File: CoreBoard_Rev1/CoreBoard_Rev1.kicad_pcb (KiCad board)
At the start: 2 copper layers, 128.8 x 84.3 mm, 90 parts, among them J1 RJ45_LED_Shielded, SW1 SW_Push, SW10 SW_Push, SW11 SW_Push, SW12 SW_Push, SW13 SW_Push, SW14 SW_Push, SW15 SW_Push, SW16 SW_SPDT, SW2 SW_Push, SW3 SW_Push, SW4 SW_Push, SW5 SW_Push, SW6 SW_Push, SW7 SW_Push, SW8 SW_Push, SW9 SW_Push, U1 Teensy4.1_DEV-16771, U2 TSR_1-2450, U4 74HC148, U5 74HC148, U6 74HC00, U7 OKI

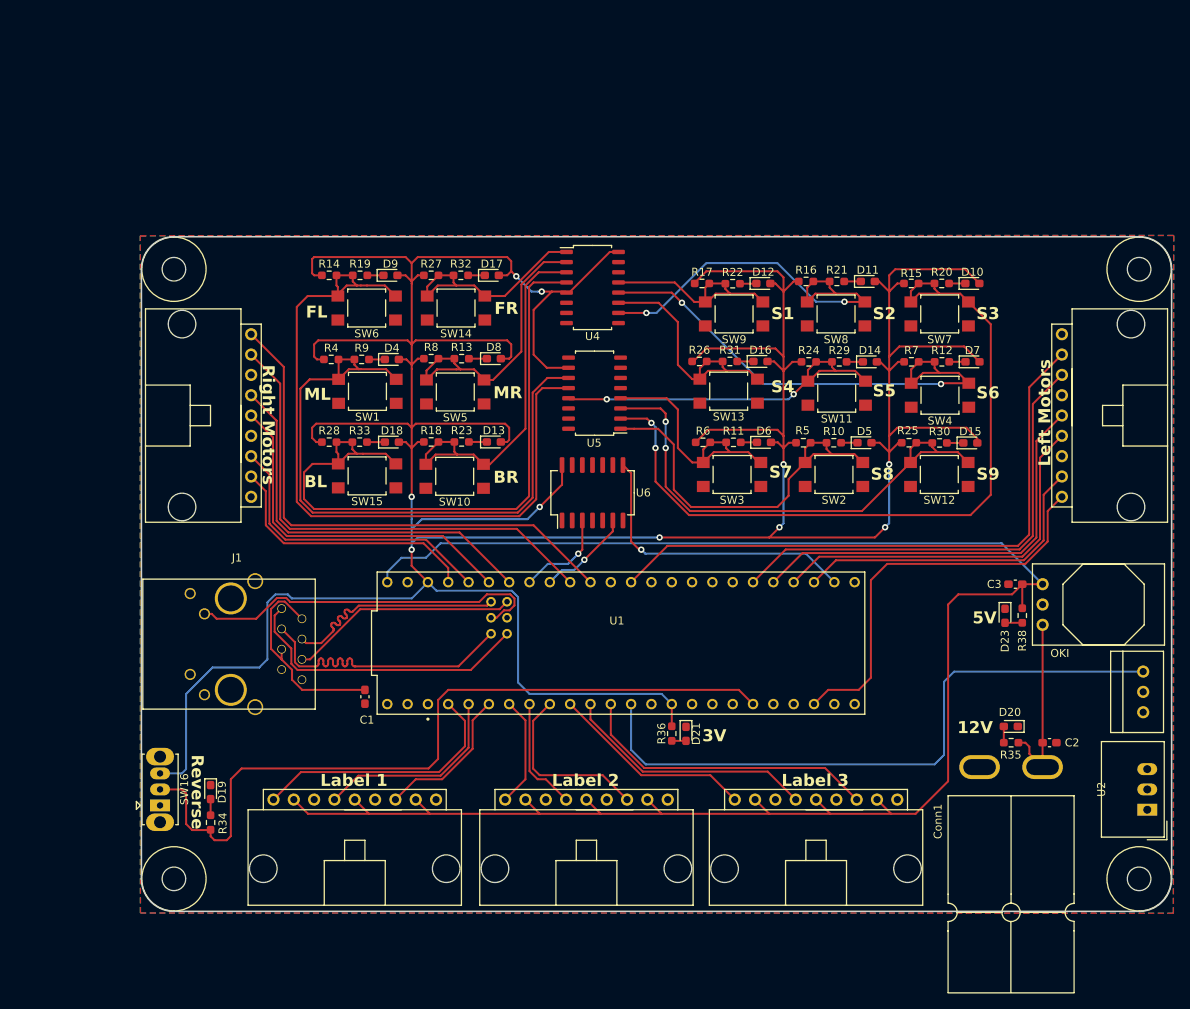
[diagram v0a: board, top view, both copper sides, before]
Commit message: connected remaining components
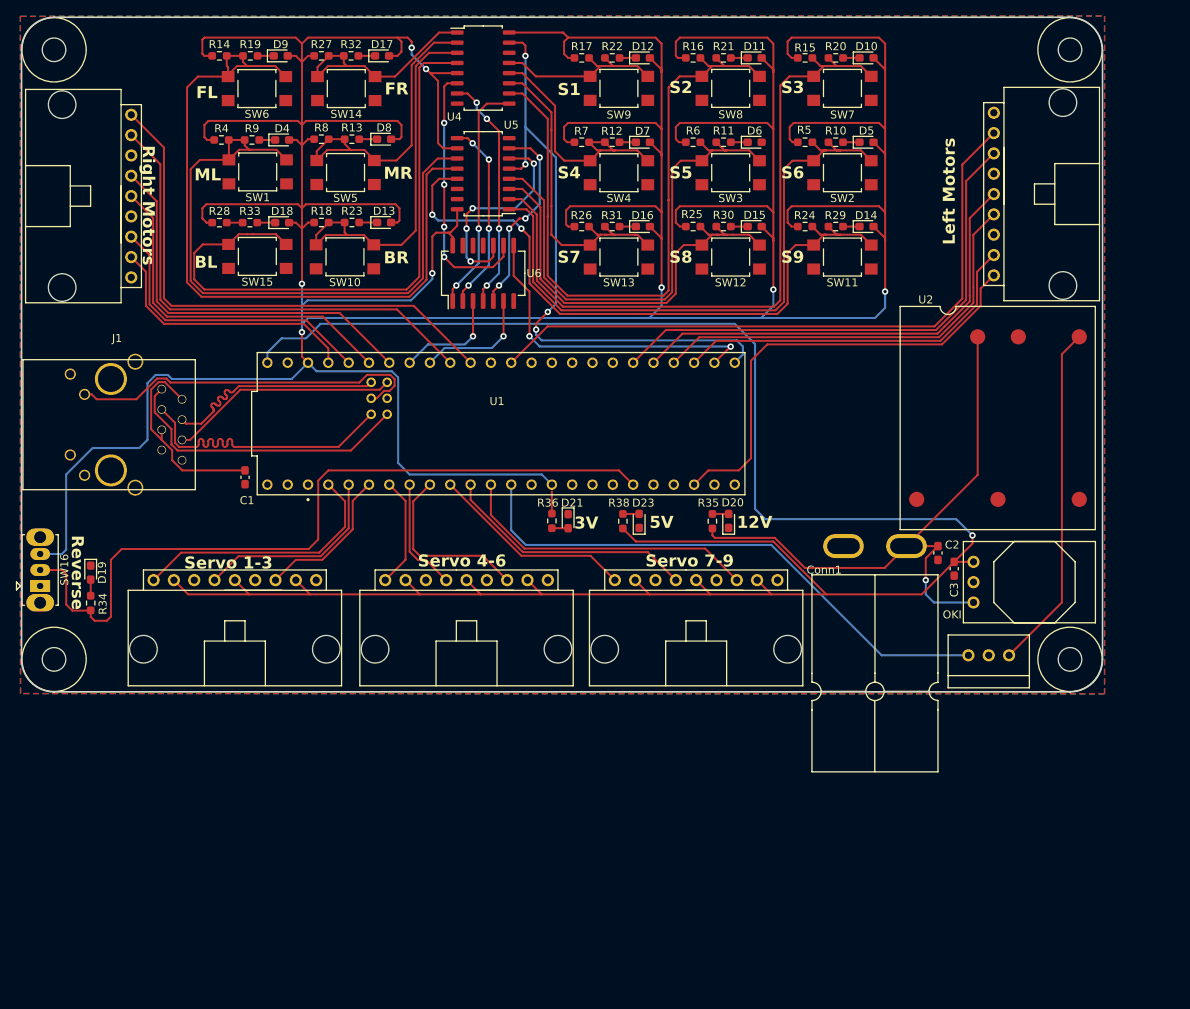
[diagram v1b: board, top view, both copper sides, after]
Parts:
- U2: footprint Converter_DCDC:Converter_DCDC_TRACO_TSR-1_THT -> MRDT_Devices:SHHD003A0A-SRZ
- moved U2 70.1 mm to (176.6, 68.4), turned to -90 degrees
- moved R38 51.3 mm to (142.0, 95.2), turned to 90 degrees
- moved R12 49.5 mm to (140.6, 47.9)
- moved R7 49.5 mm to (136.8, 47.9)
- moved D7 49.5 mm to (144.5, 47.9)
- moved SW4 48.8 mm to (141.5, 51.7)
- moved D23 47.2 mm to (144.0, 95.2), turned to 90 degrees
- moved R35 46.5 mm to (153.2, 95.2), turned to 90 degrees
- moved D20 43.6 mm to (155.2, 95.2), turned to 90 degrees
- moved R30 38.2 mm to (154.6, 58.4)
- moved R25 38.2 mm to (150.7, 58.4)
- moved D15 38.2 mm to (158.4, 58.4)
- moved SW2 37.7 mm to (169.4, 51.7)
- moved SW3 37.7 mm to (155.4, 51.7)
- moved SW12 37.7 mm to (155.4, 62.2)
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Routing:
- net +3V3: track 525.5 -> 641.1 mm, vias 10 -> 8
- net Out3: track 0.00 -> 76.7 mm, vias 0 -> 4
- net PV: track 23.5 -> 75.7 mm, vias 0 -> 1
- net Net-(U2-Vout): track 0.00 -> 43.4 mm
- net +5V: track 229.1 -> 269.5 mm, vias 0 -> 1
- net B3: track 45.0 -> 83.0 mm
- net B8: track 50.2 -> 84.7 mm, vias 2 -> 0
- net B7: track 31.0 -> 64.2 mm
- net Net-(U4-S2): track 0.00 -> 33.0 mm, vias 0 -> 4
- net B10: track 63.3 -> 31.8 mm, vias 2 -> 0
- net Net-(U4-S1): track 0.00 -> 29.7 mm, vias 0 -> 4
- net B4: track 48.5 -> 77.9 mm
- net Net-(U4-S0): track 0.00 -> 29.2 mm, vias 0 -> 2
- net Net-(U5-S2): track 0.18 -> 26.9 mm, vias 0 -> 4
- net Net-(U5-S1): track 0.00 -> 25.1 mm, vias 0 -> 4
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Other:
- board size 128.8 x 84.3 mm -> 135.1 x 84.3 mm
- board text added: "Servo 1-3"
- board text added: "Servo 4-6"
- board text added: "Servo 7-9"
- board text added: "logo here?"
- board text added: "lots of islands, make grounding better"
- board text added: "make everything more aligned generally nicer looking"
- board text added: "redo left buttons please <3"
- board text removed: "Label 1"
- board text removed: "Label 2"
- board text removed: "Label 3"
